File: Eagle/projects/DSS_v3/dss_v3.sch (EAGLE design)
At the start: 56 parts, among them IC1 MC34063AD, IC2 Atmega8a, IC3 TL431, J1 12-24V, SW1 EC12E_SW, T1 BC846, X1 PS2

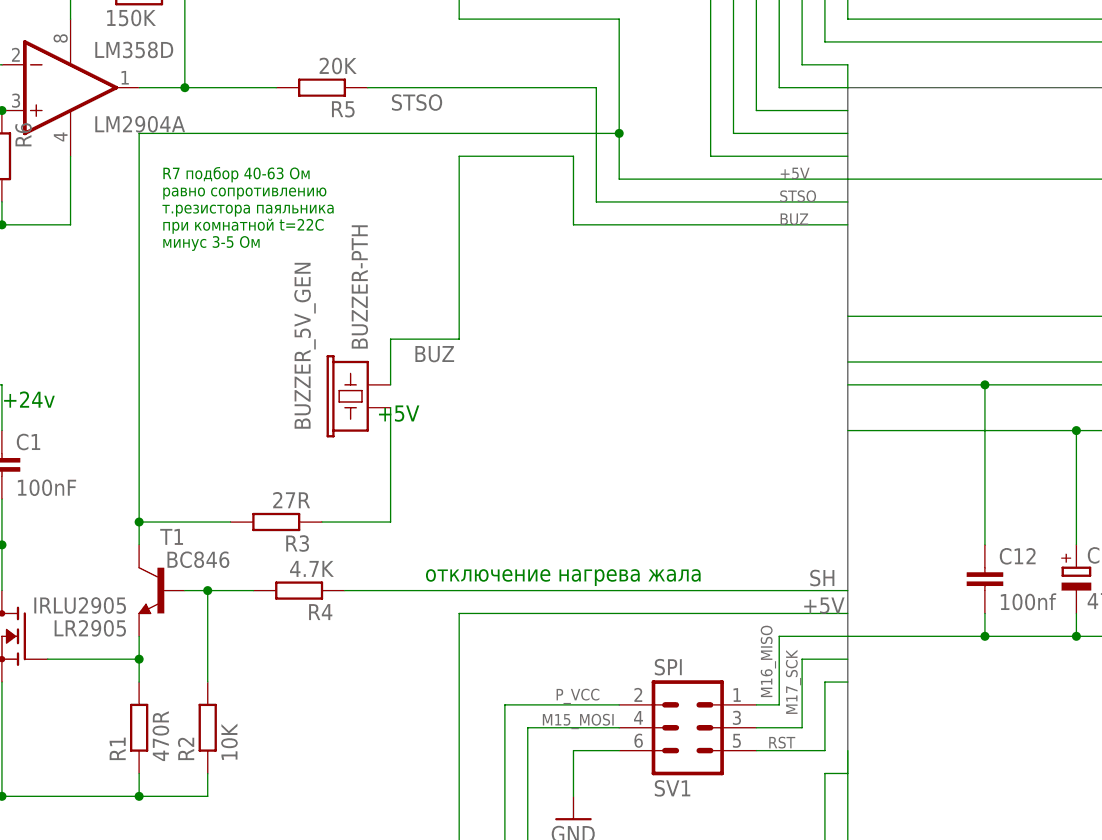
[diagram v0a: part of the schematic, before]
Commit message: update
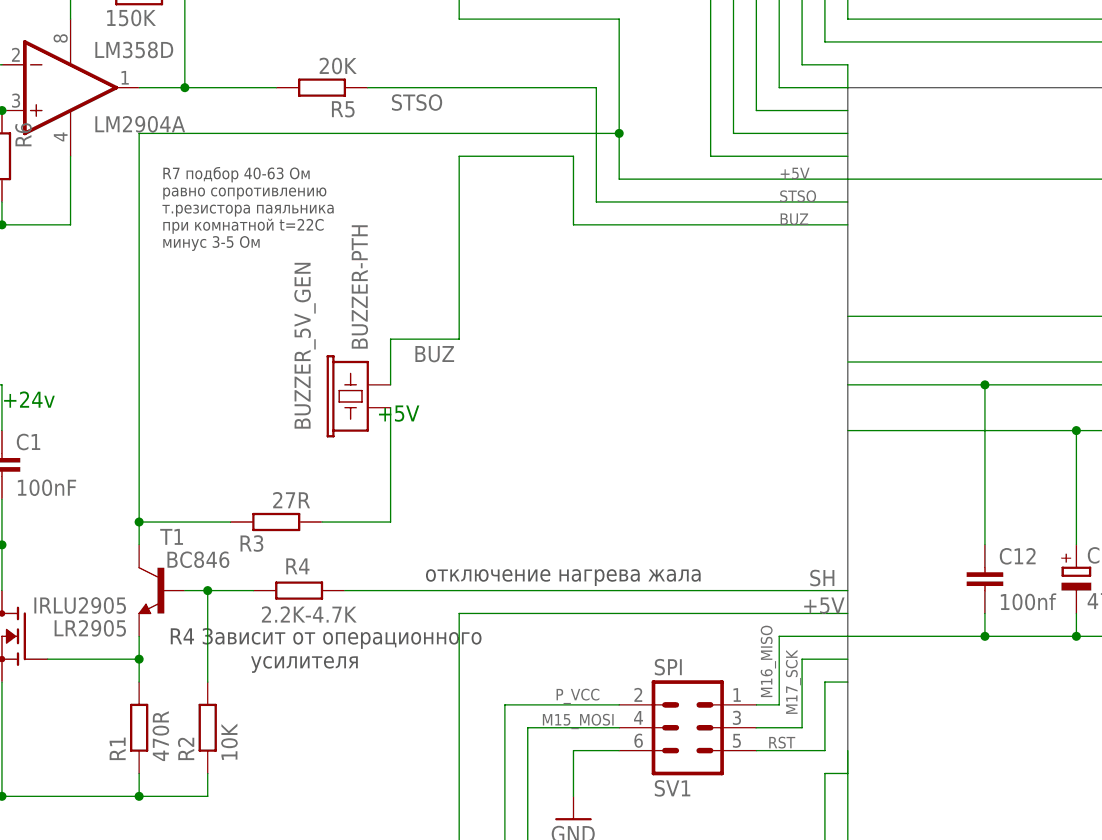
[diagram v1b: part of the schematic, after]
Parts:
- R4: value 4.7K -> 2.2K-4.7K
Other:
- note added: "R4 Зависит от операционного усилителя"
